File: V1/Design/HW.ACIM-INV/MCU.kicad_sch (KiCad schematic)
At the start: 5 parts

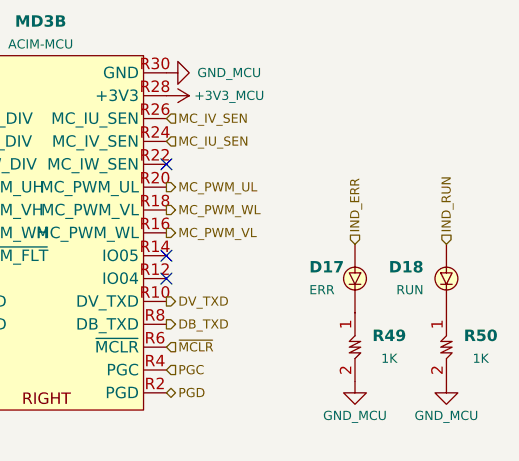
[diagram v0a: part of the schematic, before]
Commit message: V1 schematic update 21
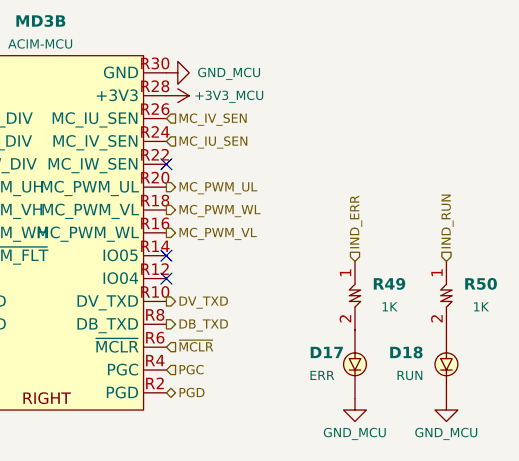
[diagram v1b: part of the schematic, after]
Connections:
- net GND_MCU: now also D17.K, D18.K; no longer R49.2, R50.2
- net IND_ERR: now also R49.1; no longer D17.A
- net IND_RUN: now also R50.1; no longer D18.A
- new net: D18.A, R50.2
- new net: D17.A, R49.2
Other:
- moved on the sheet: D17, D18, R49, R50
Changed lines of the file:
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@@
 	(hierarchical_label "IND_RUN"
 		(shape input)
-		(at 213.36 88.9 90)
+		(at 213.36 90.805 90)
 		(fields_autoplaced yes)
 		(effects
@@
 	(hierarchical_label "IND_ERR"
 		(shape input)
-		(at 203.2 88.9 90)
+		(at 203.2 90.805 90)
 		(fields_autoplaced yes)
 		(effects
@@
 	(symbol
 		(lib_id "SAMPI:RES")
-		(at 210.82 99.06 90)
+		(at 210.82 93.345 90)
 		(mirror x)
 		(unit 1)
@@
 		(dnp no)
 		(property "Reference" "R50"
-			(at 217.17 99.06 90)
+			(at 217.17 93.345 90)
 			(effects
 				(font
@@
 		)
 		(property "Value" "1K"
-			(at 217.17 101.6 90)
+			(at 217.17 95.885 90)
 			(effects
 				(font
@@
 		)
 		(property "Footprint" "SAMPI:RES0603"
-			(at 210.82 99.06 0)
+			(at 210.82 93.345 0)
 			(effects
 				(font
@@
 		)
 		(property "Datasheet" ""
-			(at 210.82 99.06 0)
+			(at 210.82 93.345 0)
 			(effects
 				(font
@@
 		)
 		(property "Description" "RES 1K OHM 5% 1/10W 0603"
-			(at 210.82 99.06 0)
+			(at 210.82 93.345 0)
 			(effects
 				(font
@@
 		)
 		(property "MFT" "YAGEO"
-			(at 210.82 99.06 0)
+			(at 210.82 93.345 0)
 			(effects
 				(font
@@
 		)
 		(property "MNP" "RC0603JR-071KL"
-			(at 210.82 99.06 0)
+			(at 210.82 93.345 0)
 			(effects
 				(font
@@
 	(symbol
 		(lib_id "SAMPI:GLED")
-		(at 210.82 90.805 90)
+		(at 210.82 100.33 90)
 		(mirror x)
 		(unit 1)
@@
 		(fields_autoplaced yes)
 		(property "Reference" "D18"
-			(at 210.82 91.4399 90)
+			(at 210.82 100.9649 90)
 			(effects
 				(font
@@
 		)
 		(property "Value" "RUN"
-			(at 210.82 93.9799 90)
+			(at 210.82 103.5049 90)
 			(effects
 				(font
@@
 		)
 		(property "Footprint" "SAMPI:LED0603"
-			(at 210.82 90.805 0)
+			(at 210.82 100.33 0)
 			(effects
 				(font
@@
 		)
 		(property "Datasheet" ""
-			(at 210.82 90.805 0)
+			(at 210.82 100.33 0)
 			(effects
 				(font
@@
 		)
 		(property "Description" "LED GREEN DIFFUSED 0603 SMD"
-			(at 210.82 90.805 0)
+			(at 210.82 100.33 0)
 			(effects
 				(font
@@
 		)
 		(property "MFT" "Harvatek"
-			(at 210.82 90.805 0)
+			(at 210.82 100.33 0)
 			(effects
 				(font
@@
 		)
 		(property "MNP" "B1911NG--20D000214U1930"
-			(at 210.82 90.805 0)
+			(at 210.82 100.33 0)
 			(effects
 				(font
@@
 	(symbol
 		(lib_id "SAMPI:GND_MCU")
-		(at 203.2 104.14 0)
+		(at 203.2 106.045 0)
 		(unit 1)
 		(exclude_from_sim no)
@@
 		(dnp no)
 		(property "Reference" "#PWR0170"
-			(at 203.2 110.49 0)
+			(at 203.2 112.395 0)
 			(effects
 				(font
@@
 		)
 		(property "Value" "GND_MCU"
-			(at 203.2 107.95 0)
+			(at 203.2 109.855 0)
 			(effects
 				(font
@@
 		)
 		(property "Footprint" ""
-			(at 203.2 104.14 0)
+			(at 203.2 106.045 0)
 			(effects
 				(font
@@
 		)
 		(property "Datasheet" ""
-			(at 203.2 104.14 0)
+			(at 203.2 106.045 0)
 			(effects
 				(font
@@
 		)
 		(property "Description" "Power symbol creates a global label with name \"GND\" , ground"
-			(at 203.2 104.14 0)
+			(at 203.2 106.045 0)
 			(effects
 				(font
@@
 	(symbol
 		(lib_id "SAMPI:GND_MCU")
-		(at 213.36 104.14 0)
+		(at 213.36 106.045 0)
 		(unit 1)
 		(exclude_from_sim no)
@@
 		(dnp no)
 		(property "Reference" "#PWR0171"
-			(at 213.36 110.49 0)
+			(at 213.36 112.395 0)
 			(effects
 				(font
@@
 		)
 		(property "Value" "GND_MCU"
-			(at 213.36 107.95 0)
+			(at 213.36 109.855 0)
 			(effects
 				(font
@@
 		)
 		(property "Footprint" ""
-			(at 213.36 104.14 0)
+			(at 213.36 106.045 0)
 			(effects
 				(font
@@
 		)
 		(property "Datasheet" ""
-			(at 213.36 104.14 0)
+			(at 213.36 106.045 0)
 			(effects
 				(font
@@
 		)
 		(property "Description" "Power symbol creates a global label with name \"GND\" , ground"
-			(at 213.36 104.14 0)
+			(at 213.36 106.045 0)
 			(effects
 				(font
@@
 	(symbol
 		(lib_id "SAMPI:RES")
-		(at 200.66 99.06 90)
+		(at 200.66 93.345 90)
 		(mirror x)
 		(unit 1)
@@
 		(dnp no)
 		(property "Reference" "R49"
-			(at 207.01 99.06 90)
+			(at 207.01 93.345 90)
 			(effects
 				(font
@@
 		)
 		(property "Value" "1K"
-			(at 207.01 101.6 90)
+			(at 207.01 95.885 90)
 			(effects
 				(font
@@
 		)
 		(property "Footprint" "SAMPI:RES0603"
-			(at 200.66 99.06 0)
+			(at 200.66 93.345 0)
 			(effects
 				(font
@@
 		)
 		(property "Datasheet" ""
-			(at 200.66 99.06 0)
+			(at 200.66 93.345 0)
 			(effects
 				(font
@@
 		)
 		(property "Description" "RES 1K OHM 5% 1/10W 0603"
-			(at 200.66 99.06 0)
+			(at 200.66 93.345 0)
 			(effects
 				(font
@@
 		)
 		(property "MFT" "YAGEO"
-			(at 200.66 99.06 0)
+			(at 200.66 93.345 0)
 			(effects
 				(font
@@
 		)
 		(property "MNP" "RC0603JR-071KL"
-			(at 200.66 99.06 0)
+			(at 200.66 93.345 0)
 			(effects
 				(font
@@
 	(symbol
 		(lib_id "SAMPI:RLED")
-		(at 207.645 91.44 270)
+		(at 207.645 100.965 270)
 		(unit 1)
 		(exclude_from_sim no)
@@
 		(dnp no)
 		(property "Reference" "D17"
-			(at 198.12 91.44 90)
+			(at 198.12 100.965 90)
 			(effects
 				(font
@@
 		)
 		(property "Value" "ERR"
-			(at 198.12 93.98 90)
+			(at 198.12 103.505 90)
 			(effects
 				(font
@@
 		)
 		(property "Footprint" "SAMPI:LED0603"
-			(at 207.645 91.44 0)
+			(at 207.645 100.965 0)
 			(effects
 				(font
@@
 		)
 		(property "Datasheet" ""
-			(at 207.645 91.44 0)
+			(at 207.645 100.965 0)
 			(effects
 				(font
@@
 		)
 		(property "Description" "LED RED DIFFUSED 0603 SMD"
-			(at 207.645 91.44 0)
+			(at 207.645 100.965 0)
 			(effects
 				(font
@@
 		)
 		(property "MFT" "Harvatek"
-			(at 207.645 91.44 0)
+			(at 207.645 100.965 0)
 			(effects
 				(font
@@
 		)
 		(property "MNP" "B1911USD-20D000114U1930"
-			(at 207.645 91.44 0)
-			(effects
-				(font
+			(at 207.645 100.965 0)
+			(effects
+				(font
